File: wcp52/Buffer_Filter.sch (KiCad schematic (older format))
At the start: 18 parts, among them Q10 BFR540, Q8 MMBT3904, Q9 BFR540

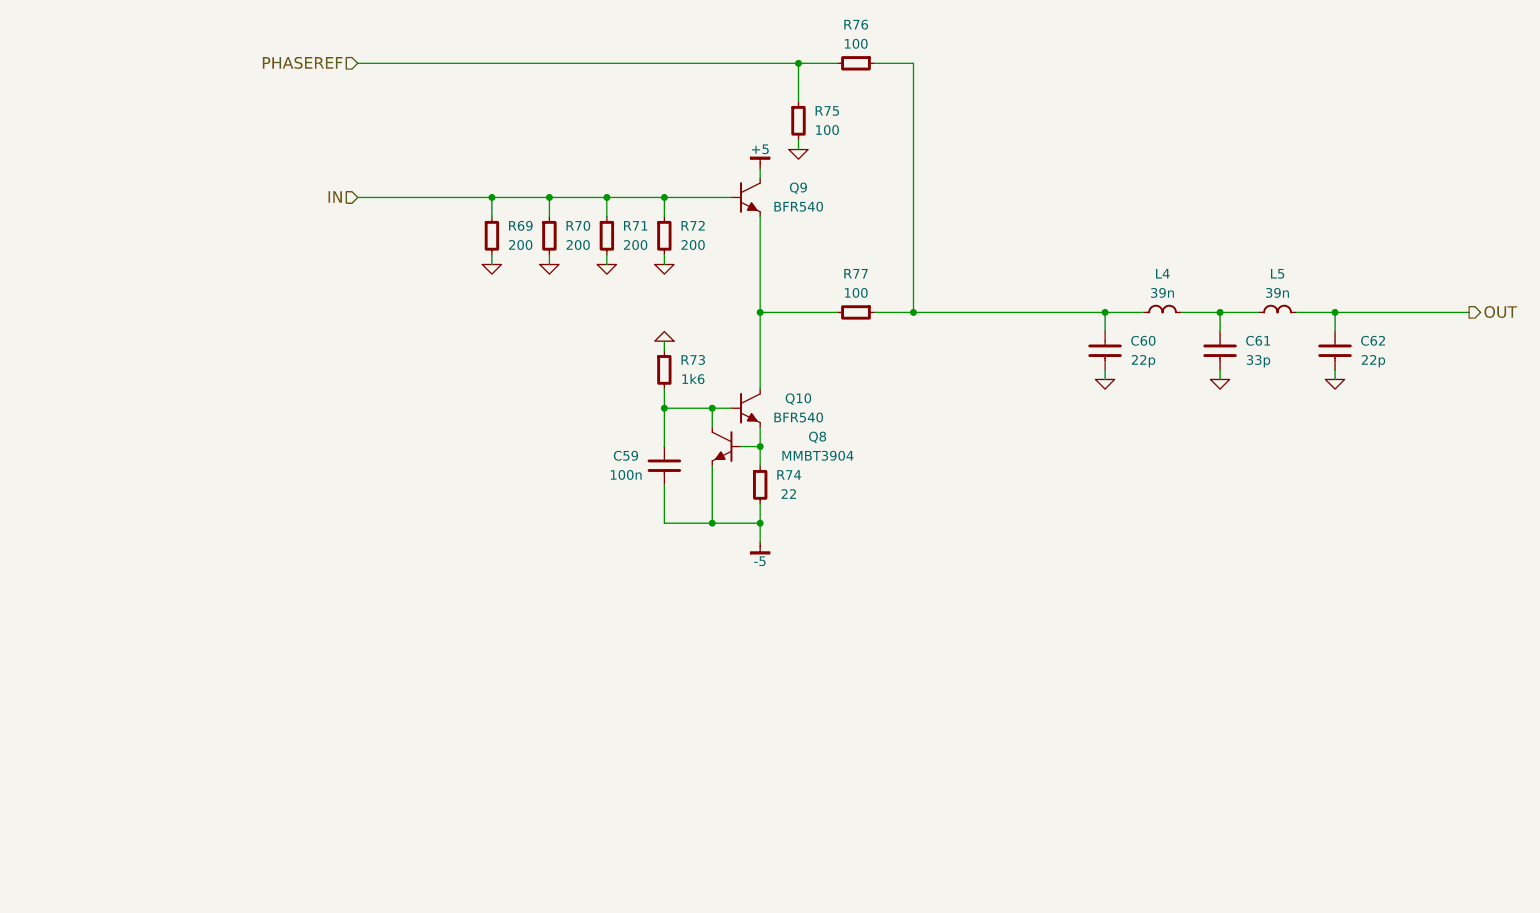
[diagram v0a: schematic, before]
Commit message: Schematic touchups
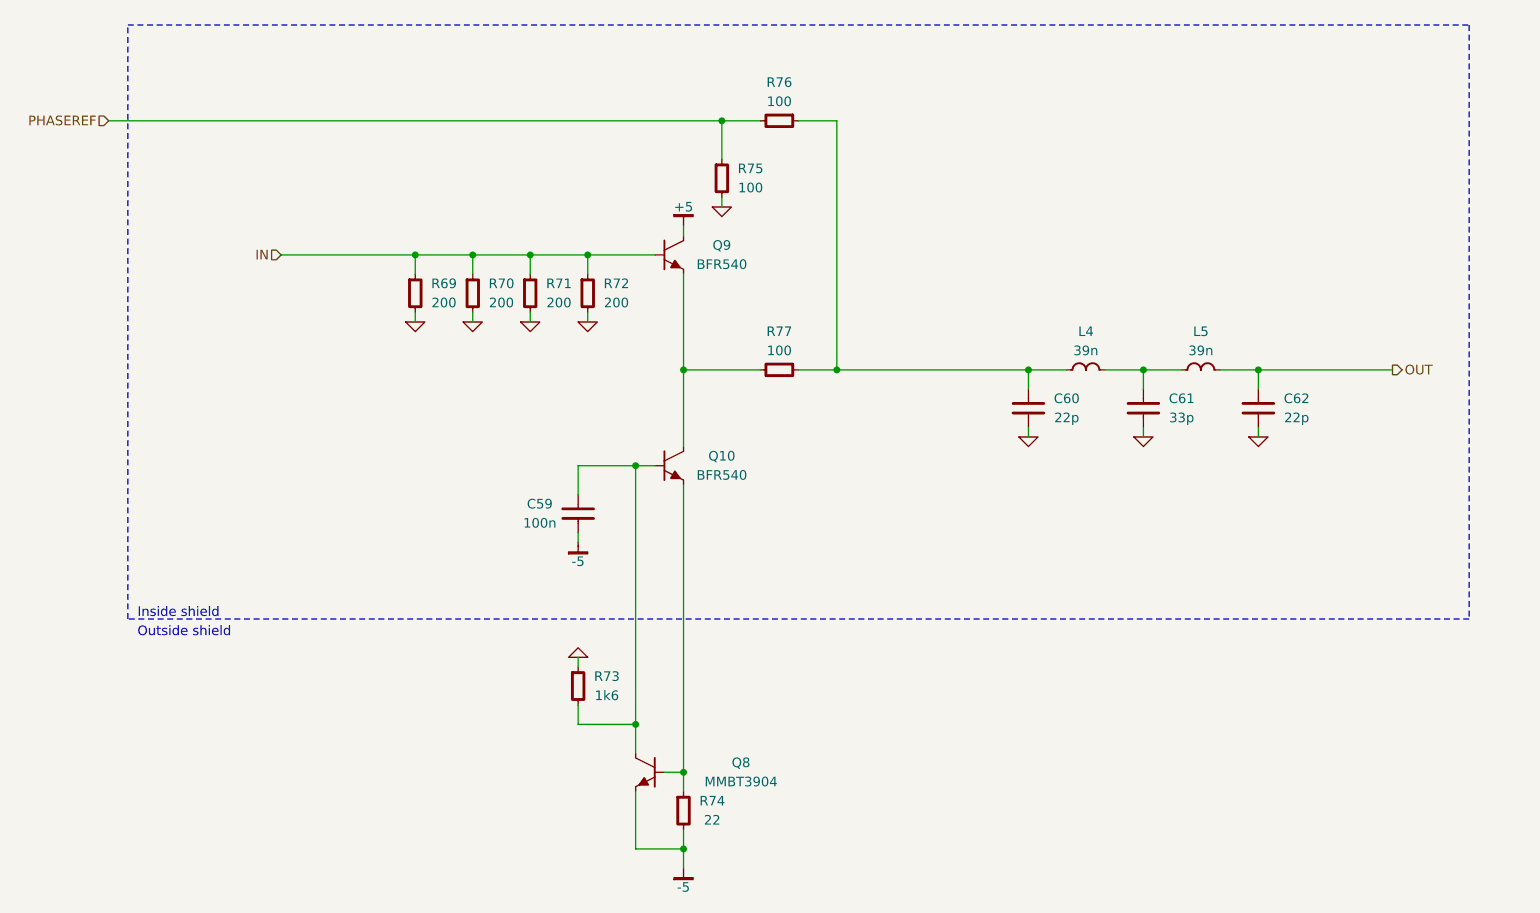
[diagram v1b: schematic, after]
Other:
- note added: "Inside shield"
- note added: "Outside shield"
- moved on the sheet: C59, C60, C61, C62, L4, L5, Q10, Q8, Q9, R69, R70, R71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
